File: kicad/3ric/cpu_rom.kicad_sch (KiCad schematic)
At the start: 15 parts, among them J1_AND 74LS08, J3_DEV_DECODE 74LS154, K1_CPU 6502-library_65C02S-2, K2_ROM SST39SF040

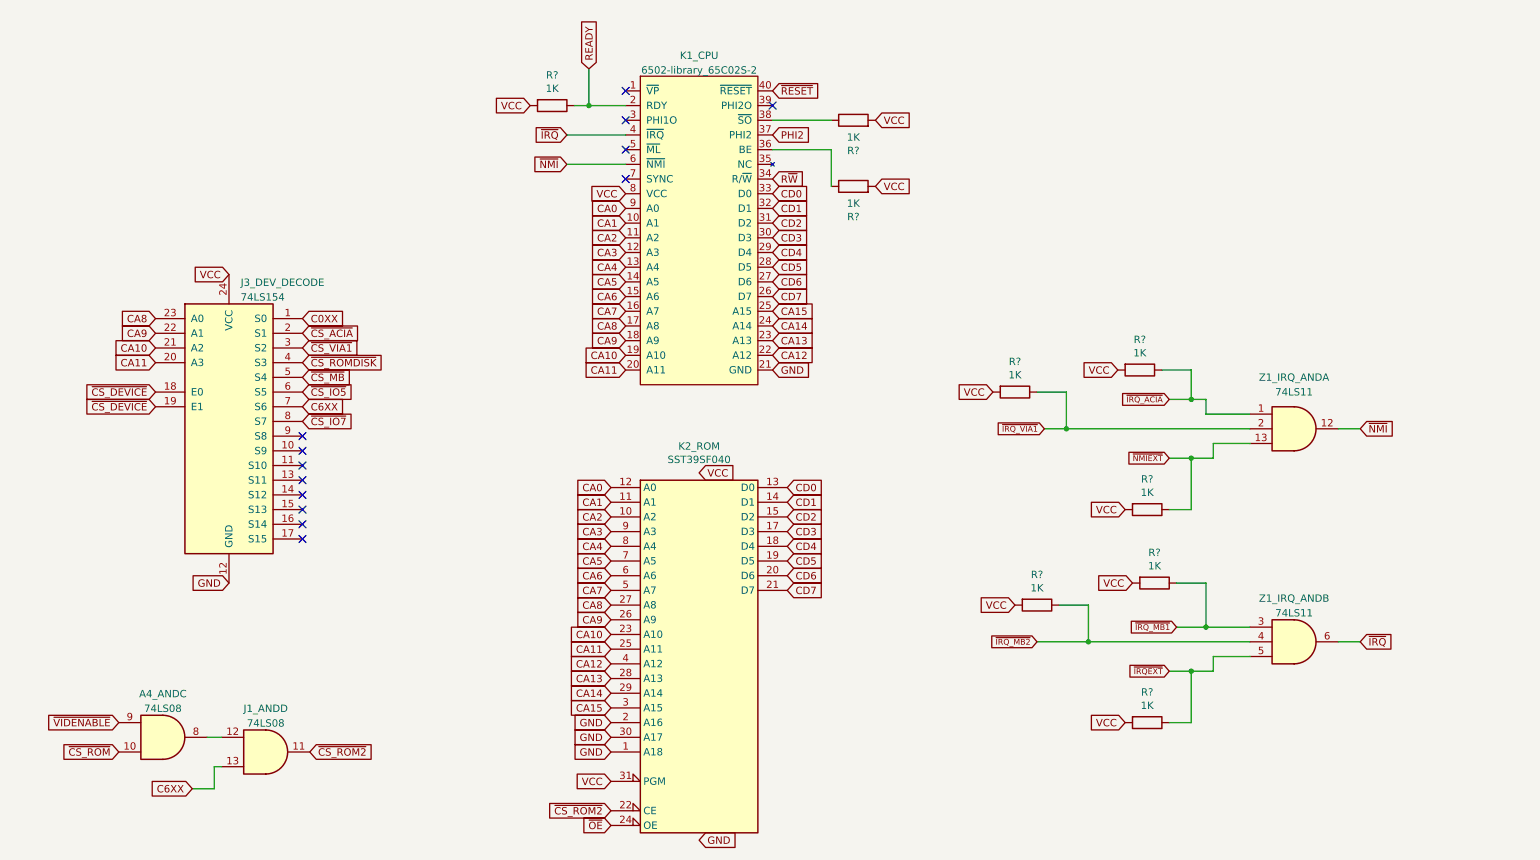
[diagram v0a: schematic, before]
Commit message: cleaning up of the schematic
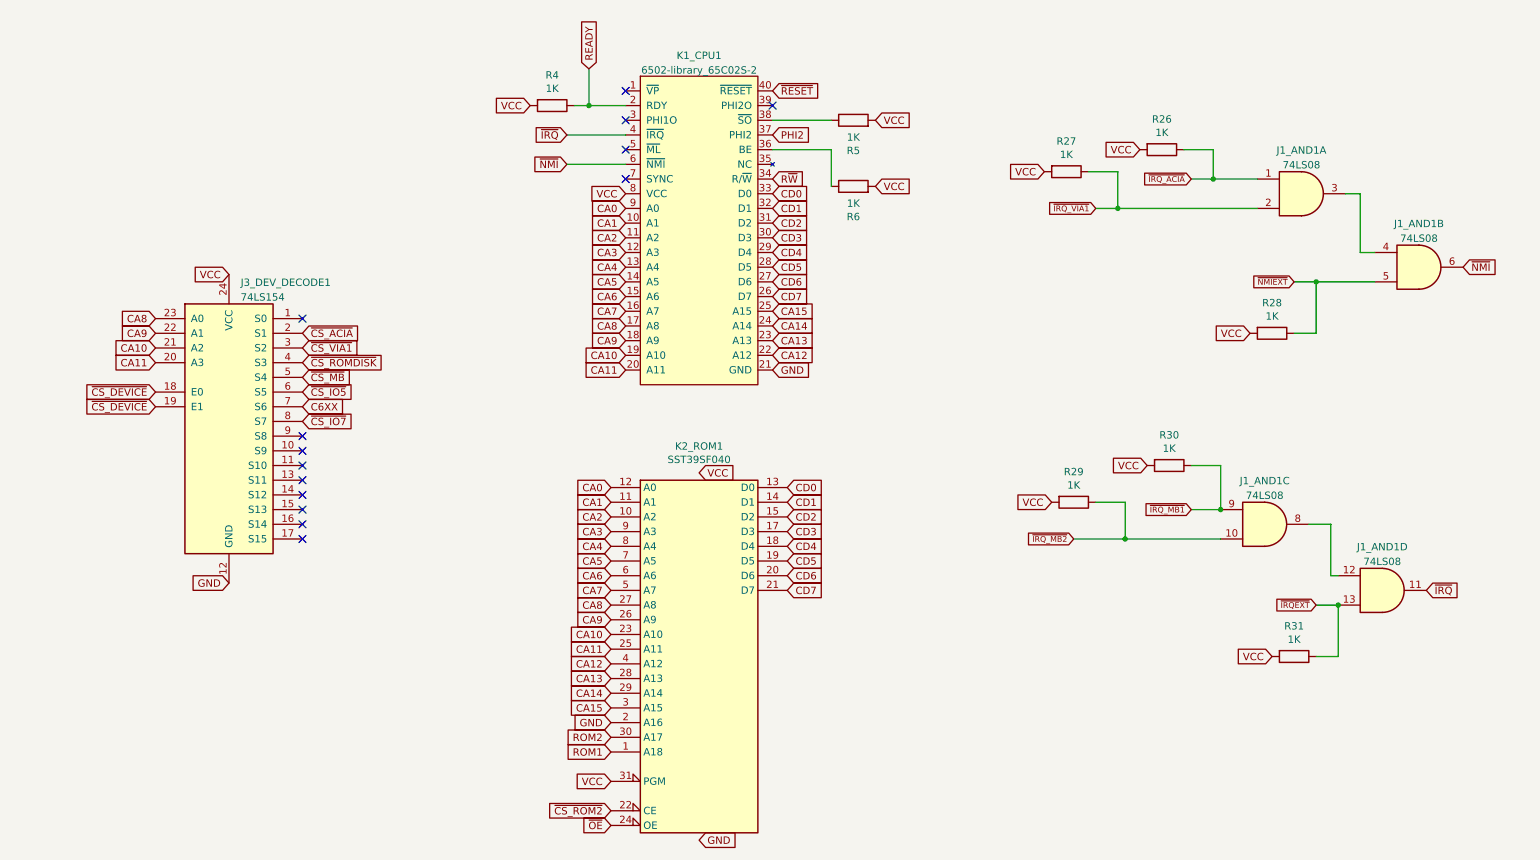
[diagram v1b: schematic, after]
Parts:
- removed A4_AND, J1_AND: 74LS08, symbol 74xx:74LS08
- removed R? (x6): 1K, Resistor_THT:R_Axial_DIN0207_L6.3mm_D2.5mm_P7.62mm_Horizontal, symbol Device:R
- removed Z1_IRQ_AND: 74LS11, symbol 74xx:74LS11
- added J1_AND1: 74LS08, Package_DIP:DIP-14_W7.62mm_Socket, symbol 74xx:74LS08
- added R26, R27, R28, R29, R30, R31: 1K, Resistor_THT:R_Axial_DIN0207_L6.3mm_D2.5mm_P7.62mm_Horizontal, symbol Device:R
- gave numbers to parts that had none: 3
- renumbered J3_DEV_DECODE to J3_DEV_DECODE1, K1_CPU to K1_CPU1, K2_ROM to K2_ROM1
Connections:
- net GND: no longer K2_ROM1.1 (A18), K2_ROM1.30 (A17)
- net VCC: now also R26.2, R27.2, R28.2, R29.2, R30.2, R31.2
- net ~{IRQEXT}: now also J1_AND1.13, R31.1
- net ~{IRQ_ACIA}: now also J1_AND1.1, R26.1
- net ~{IRQ_MB1}: now also J1_AND1.9, R30.1
- net ~{IRQ_MB2}: now also J1_AND1.10, R29.1
- net ~{IRQ_VIA1}: now also J1_AND1.2, R27.1
- net ~{IRQ}: now also J1_AND1.11
- net ~{NMIEXT}: now also J1_AND1.5, R28.1
- net ~{NMI}: now also J1_AND1.6
- net C0XX: no longer names the net of J3_DEV_DECODE1.1 (S0)
- new net: J1_AND1.3, J1_AND1.4
- new net: J1_AND1.12, J1_AND1.8
- new net ROM1: K2_ROM1.1 (A18)
- new net ROM2: K2_ROM1.30 (A17)
- no-connect marks 13 -> 14
